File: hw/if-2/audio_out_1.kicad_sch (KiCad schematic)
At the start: 0 parts

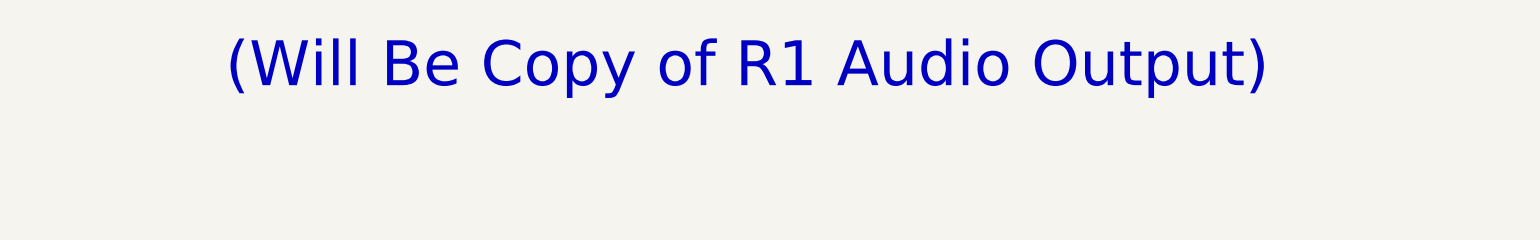
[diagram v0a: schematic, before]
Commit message: First draft of schematic
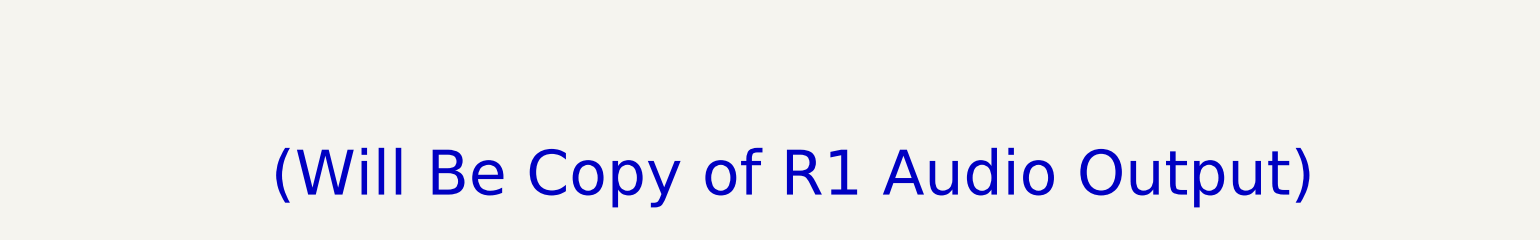
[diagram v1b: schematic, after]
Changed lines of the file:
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@@
 	(text "(Will Be Copy of R1 Audio Output)"
 		(exclude_from_sim no)
-		(at 141.732 90.932 0)
+		(at 146.812 103.124 0)
 		(effects
 			(font
